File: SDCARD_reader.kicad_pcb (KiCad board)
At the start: 2 copper layers, 20 x 30 mm, 16 parts, among them J1 USB_B_Micro, U1 GL827L, Y1 O12M

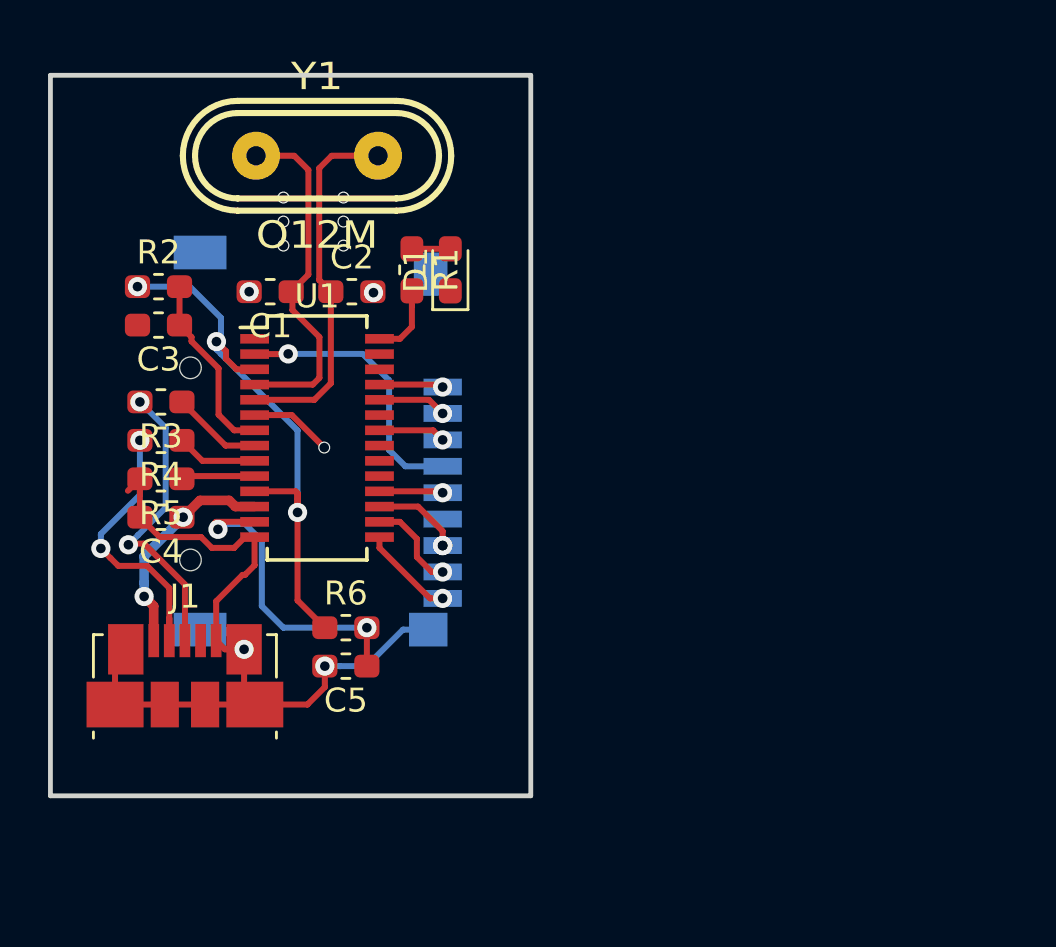
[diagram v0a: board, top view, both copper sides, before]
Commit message: update,
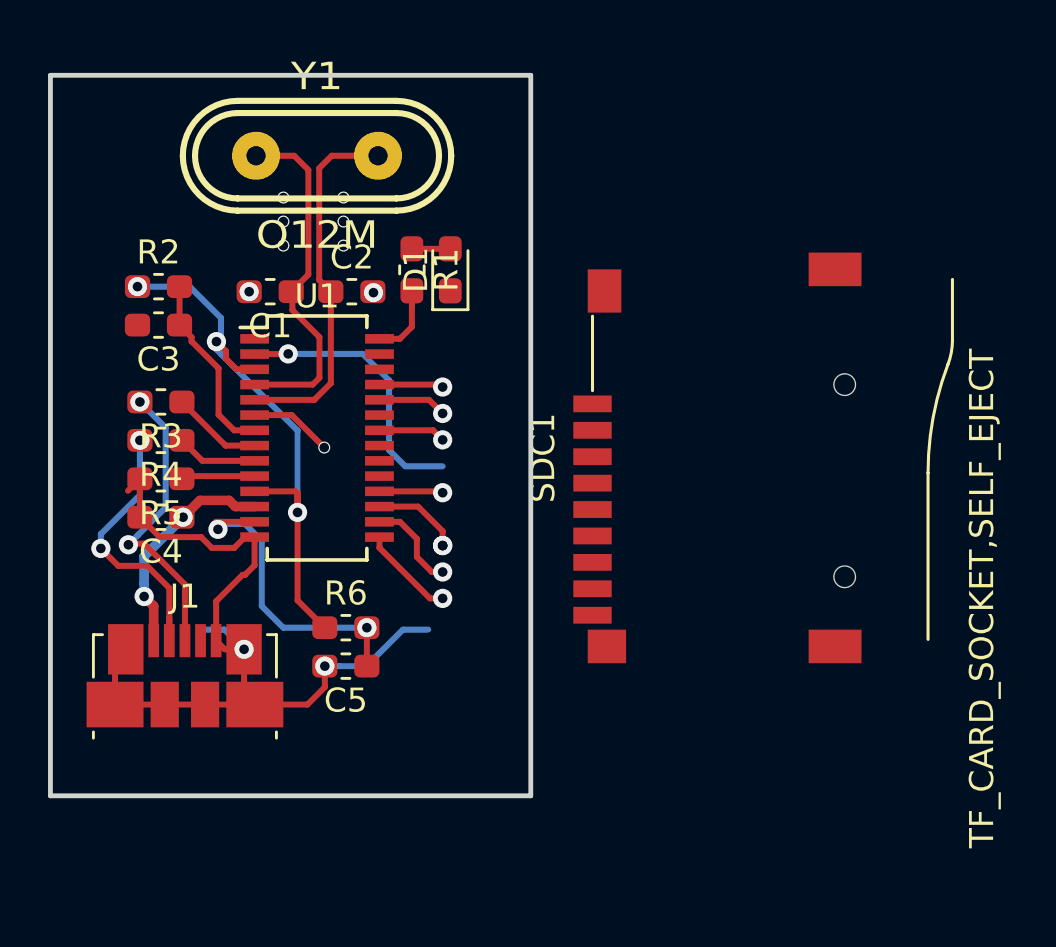
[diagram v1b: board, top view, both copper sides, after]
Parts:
- SDC1: moved to F.Cu
- moved SDC1 16.9 mm to (57.9, 37.2)
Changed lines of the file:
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@@
     )
   )
-  (module footprint-lib:SUNTECH_ST-TF-003A (layer B.Cu)
-    (at 41 36.5 90)
+  (module footprint-lib:SUNTECH_ST-TF-003A (layer F.Cu)
+    (at 57.9 37.2 90)
     (attr smd)
-    (fp_text reference SDC1 (at 1.27 7.38873 90) (layer B.SilkS)
-      (effects (font (size 1.0005 1.0005) (thickness 0.05)) (justify mirror))
+    (fp_text reference SDC1 (at 1.27 -7.38873 90) (layer F.SilkS)
+      (effects (font (size 1.0005 1.0005) (thickness 0.05)))
     )
-    (fp_text value TF_CARD_SOCKET,SELF_EJECT (at -4.58364 -10.8855 90) (layer B.SilkS)
-      (effects (font (size 1.00188 1.00188) (thickness 0.05)) (justify mirror))
+    (fp_text value TF_CARD_SOCKET,SELF_EJECT (at -4.58364 10.8855 90) (layer F.SilkS)
+      (effects (font (size 1.00188 1.00188) (thickness 0.05)))
     )
-    (fp_line (start 8.699 4.187) (end 8.699 -9.656) (layer Dwgs.User) (width 0.127))
-    (fp_line (start 8.699 -9.656) (end 6.1679 -9.656) (layer B.SilkS) (width 0.127))
-    (fp_arc (start 6.16785 -6.8474) (end 5.168 -9.472) (angle 20.8) (layer B.SilkS) (width 0.127))
-    (fp_arc (start 0.646878 -21.34) (end 0.6469 -8.64) (angle -20.8) (layer B.SilkS) (width 0.127))
-    (fp_line (start 0.6469 -8.64) (end -6.287 -8.64) (layer B.SilkS) (width 0.127))
-    (fp_line (start -6.287 -8.64) (end -6.287 5.33) (layer Dwgs.User) (width 0.127))
-    (fp_line (start -6.287 5.33) (end 7.302 5.33) (layer Dwgs.User) (width 0.127))
-    (fp_line (start 7.302 5.33) (end 7.302 4.187) (layer Dwgs.User) (width 0.127))
-    (fp_line (start 7.302 4.187) (end 8.699 4.187) (layer Dwgs.User) (width 0.127))
-    (fp_poly (pts (xy 4.17167 0.92833) (xy 4.17167 -1.07304) (xy -4.83304 -1.07304) (xy -4.83304 0.92833)) (layer Dwgs.User) (width 0))
-    (fp_line (start 7.17 5.33) (end 4.07 5.33) (layer B.SilkS) (width 0.127))
-    (fp_line (start -7.75 6.5) (end 10.25 6.5) (layer Eco1.User) (width 0.127))
-    (fp_line (start 10.25 6.5) (end 10.25 -10) (layer Eco1.User) (width 0.127))
-    (fp_line (start 10.25 -10) (end -7.75 -10) (layer Eco1.User) (width 0.127))
-    (fp_line (start -7.75 -10) (end -7.75 6.5) (layer Eco1.User) (width 0.127))
-    (pad 1 smd rect (at 3.52 5.33 180) (size 1.6 0.7) (layers B.Cu B.Paste B.Mask)
+    (fp_line (start 8.699 -4.187) (end 8.699 9.656) (layer Dwgs.User) (width 0.127))
+    (fp_line (start 8.699 9.656) (end 6.1679 9.656) (layer F.SilkS) (width 0.127))
+    (fp_arc (start 6.16785 6.8474) (end 5.168 9.472) (angle -20.8) (layer F.SilkS) (width 0.127))
+    (fp_arc (start 0.646878 21.34) (end 0.6469 8.64) (angle 20.8) (layer F.SilkS) (width 0.127))
+    (fp_line (start 0.6469 8.64) (end -6.287 8.64) (layer F.SilkS) (width 0.127))
+    (fp_line (start -6.287 8.64) (end -6.287 -5.33) (layer Dwgs.User) (width 0.127))
+    (fp_line (start -6.287 -5.33) (end 7.302 -5.33) (layer Dwgs.User) (width 0.127))
+    (fp_line (start 7.302 -5.33) (end 7.302 -4.187) (layer Dwgs.User) (width 0.127))
+    (fp_line (start 7.302 -4.187) (end 8.699 -4.187) (layer Dwgs.User) (width 0.127))
+    (fp_poly (pts (xy 4.17167 -0.92833) (xy 4.17167 1.07304) (xy -4.83304 1.07304) (xy -4.83304 -0.92833)) (layer Dwgs.User) (width 0))
+    (fp_line (start 7.17 -5.33) (end 4.07 -5.33) (layer F.SilkS) (width 0.127))
+    (fp_line (start -7.75 -6.5) (end 10.25 -6.5) (layer Eco1.User) (width 0.127))
+    (fp_line (start 10.25 -6.5) (end 10.25 10) (layer Eco1.User) (width 0.127))
+    (fp_line (start 10.25 10) (end -7.75 10) (layer Eco1.User) (width 0.127))
+    (fp_line (start -7.75 10) (end -7.75 -6.5) (layer Eco1.User) (width 0.127))
+    (pad 1 smd rect (at 3.52 -5.33) (size 1.6 0.7) (layers F.Cu F.Paste F.Mask)
       (net 3 "Net-(RN1-Pad3)"))
-    (pad 2 smd rect (at 2.42 5.33 180) (size 1.6 0.7) (layers B.Cu B.Paste B.Mask)
+    (pad 2 smd rect (at 2.42 -5.33) (size 1.6 0.7) (layers F.Cu F.Paste F.Mask)
       (net 4 "Net-(RN1-Pad4)"))
-    (pad 3 smd rect (at 1.32 5.33 180) (size 1.6 0.7) (layers B.Cu B.Paste B.Mask)
+    (pad 3 smd rect (at 1.32 -5.33) (size 1.6 0.7) (layers F.Cu F.Paste F.Mask)
       (net 5 "Net-(SDC1-Pad3)"))
-    (pad 4 smd rect (at 0.22 5.33 180) (size 1.6 0.7) (layers B.Cu B.Paste B.Mask)
+    (pad 4 smd rect (at 0.22 -5.33) (size 1.6 0.7) (layers F.Cu F.Paste F.Mask)
       (net 6 /SD_VDD))
-    (pad 5 smd rect (at -0.88 5.33 180) (size 1.6 0.7) (layers B.Cu B.Paste B.Mask)
+    (pad 5 smd rect (at -0.88 -5.33) (size 1.6 0.7) (layers F.Cu F.Paste F.Mask)
       (net 7 "Net-(SDC1-Pad5)"))
-    (pad 6 smd rect (at -1.98 5.33 180) (size 1.6 0.7) (layers B.Cu B.Paste B.Mask)
+    (pad 6 smd rect (at -1.98 -5.33) (size 1.6 0.7) (layers F.Cu F.Paste F.Mask)
       (net 8 "Net-(SDC1-Pad6)"))
-    (pad 7 smd rect (at -3.08 5.33 180) (size 1.6 0.7) (layers B.Cu B.Paste B.Mask)
+    (pad 7 smd rect (at -3.08 -5.33) (size 1.6 0.7) (layers F.Cu F.Paste F.Mask)
       (net 9 "Net-(RN1-Pad2)"))
-    (pad 8 smd rect (at -4.18 5.33 180) (size 1.6 0.7) (layers B.Cu B.Paste B.Mask)
+    (pad 8 smd rect (at -4.18 -5.33) (size 1.6 0.7) (layers F.Cu F.Paste F.Mask)
       (net 10 "Net-(RN1-Pad1)"))
-    (pad 9 smd rect (at -5.28 5.33 180) (size 1.6 0.7) (layers B.Cu B.Paste B.Mask)
+    (pad 9 smd rect (at -5.28 -5.33) (size 1.6 0.7) (layers F.Cu F.Paste F.Mask)
       (net 11 "Net-(SDC1-Pad9)"))
-    (pad G smd rect (at -6.58 4.73 180) (size 1.6 1.4) (layers B.Cu B.Paste B.Mask)
+    (pad G smd rect (at -6.58 -4.73) (size 1.6 1.4) (layers F.Cu F.Paste F.Mask)
       (net 12 GND))
-    (pad G smd rect (at -6.58 -4.77 180) (size 2.2 1.4) (layers B.Cu B.Paste B.Mask)
+    (pad G smd rect (at -6.58 4.77) (size 2.2 1.4) (layers F.Cu F.Paste F.Mask)
       (net 12 GND))
-    (pad G smd rect (at 8.22 4.83 180) (size 1.4 1.8) (layers B.Cu B.Paste B.Mask)
+    (pad G smd rect (at 8.22 -4.83) (size 1.4 1.8) (layers F.Cu F.Paste F.Mask)
       (net 12 GND))
-    (pad G smd rect (at 9.12 -4.77 180) (size 2.2 1.4) (layers B.Cu B.Paste B.Mask)
+    (pad G smd rect (at 9.12 4.77) (size 2.2 1.4) (layers F.Cu F.Paste F.Mask)
       (net 12 GND))
-    (pad Hole np_thru_hole circle (at -3.68 -5.17 90) (size 0.9 0.9) (drill 0.9) (layers *.Cu *.Mask B.SilkS))
-    (pad Hole np_thru_hole circle (at 4.32 -5.17 90) (size 0.9 0.9) (drill 0.9) (layers *.Cu *.Mask B.SilkS))
+    (pad Hole np_thru_hole circle (at -3.68 5.17 90) (size 0.9 0.9) (drill 0.9) (layers *.Cu *.Mask F.SilkS))
+    (pad Hole np_thru_hole circle (at 4.32 5.17 90) (size 0.9 0.9) (drill 0.9) (layers *.Cu *.Mask F.SilkS))
   )
   (gr_line (start 50 20) (end 30 20) (layer Edge.Cuts) (width 0.2))
